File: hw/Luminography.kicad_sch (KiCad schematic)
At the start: 135 parts, among them J1 USB_C_Receptacle_PowerOnly_6P, J2 Conn_01x04, Q1 2N7002, SW1 SW_Push, SW2 SW_Push, U1 LTC4054ES5-4.2, U10 MAX98357AETE+, U100 BH1750FVI-TR, U101 BH1750FVI-TR, U102 BH1750FVI-TR, U103 BH1750FVI-TR, U104 BH1750FVI-TR, U105 BH1750FVI-TR, U106 BH1750FVI-TR, U107 BH1750FVI-TR, U108 BH1750FVI-TR, U109 BH1750FVI-TR, U110 BH1750FVI-TR, U111 BH1750FVI-TR, U112 BH1750FVI-TR, U113 BH1750FVI-TR, U114 BH1750FVI-TR, U115 BH1750FVI-TR, U116 BH1750FVI-TR, U117 BH1750FVI-TR, U118 BH1750FVI-TR, U119 BH1750FVI-TR, U120 BH1750FVI-TR, U121 BH1750FVI-TR, U122 BH1750FVI-TR, U123 BH1750FVI-TR, U2 XS3A1T3157GMX, U200 HD107S, U201 HD107S, U202 HD107S, U203 HD107S, U204 HD107S, U205 HD107S, U206 HD107S, U207 HD107S, U208 HD107S, U209 HD107S, U210 HD107S, U211 HD107S, U212 HD107S, U213 HD107S, U214 HD107S, U215 HD107S, U216 HD107S, U217 HD107S, U218 HD107S, U219 HD107S, U220 HD107S, U221 HD107S, U222 HD107S, U223 HD107S, U3 SPX3819M5-L-3-3, U4 MAX17048G+T10, U5 STM32G030K6Tx, U51 STM32G030C8Tx, U6 ZJY128R-IG01, U7 W25Q16JVUXIQ, U8 BMI270, U9 MMC5603NJ, X1 12.288MHz

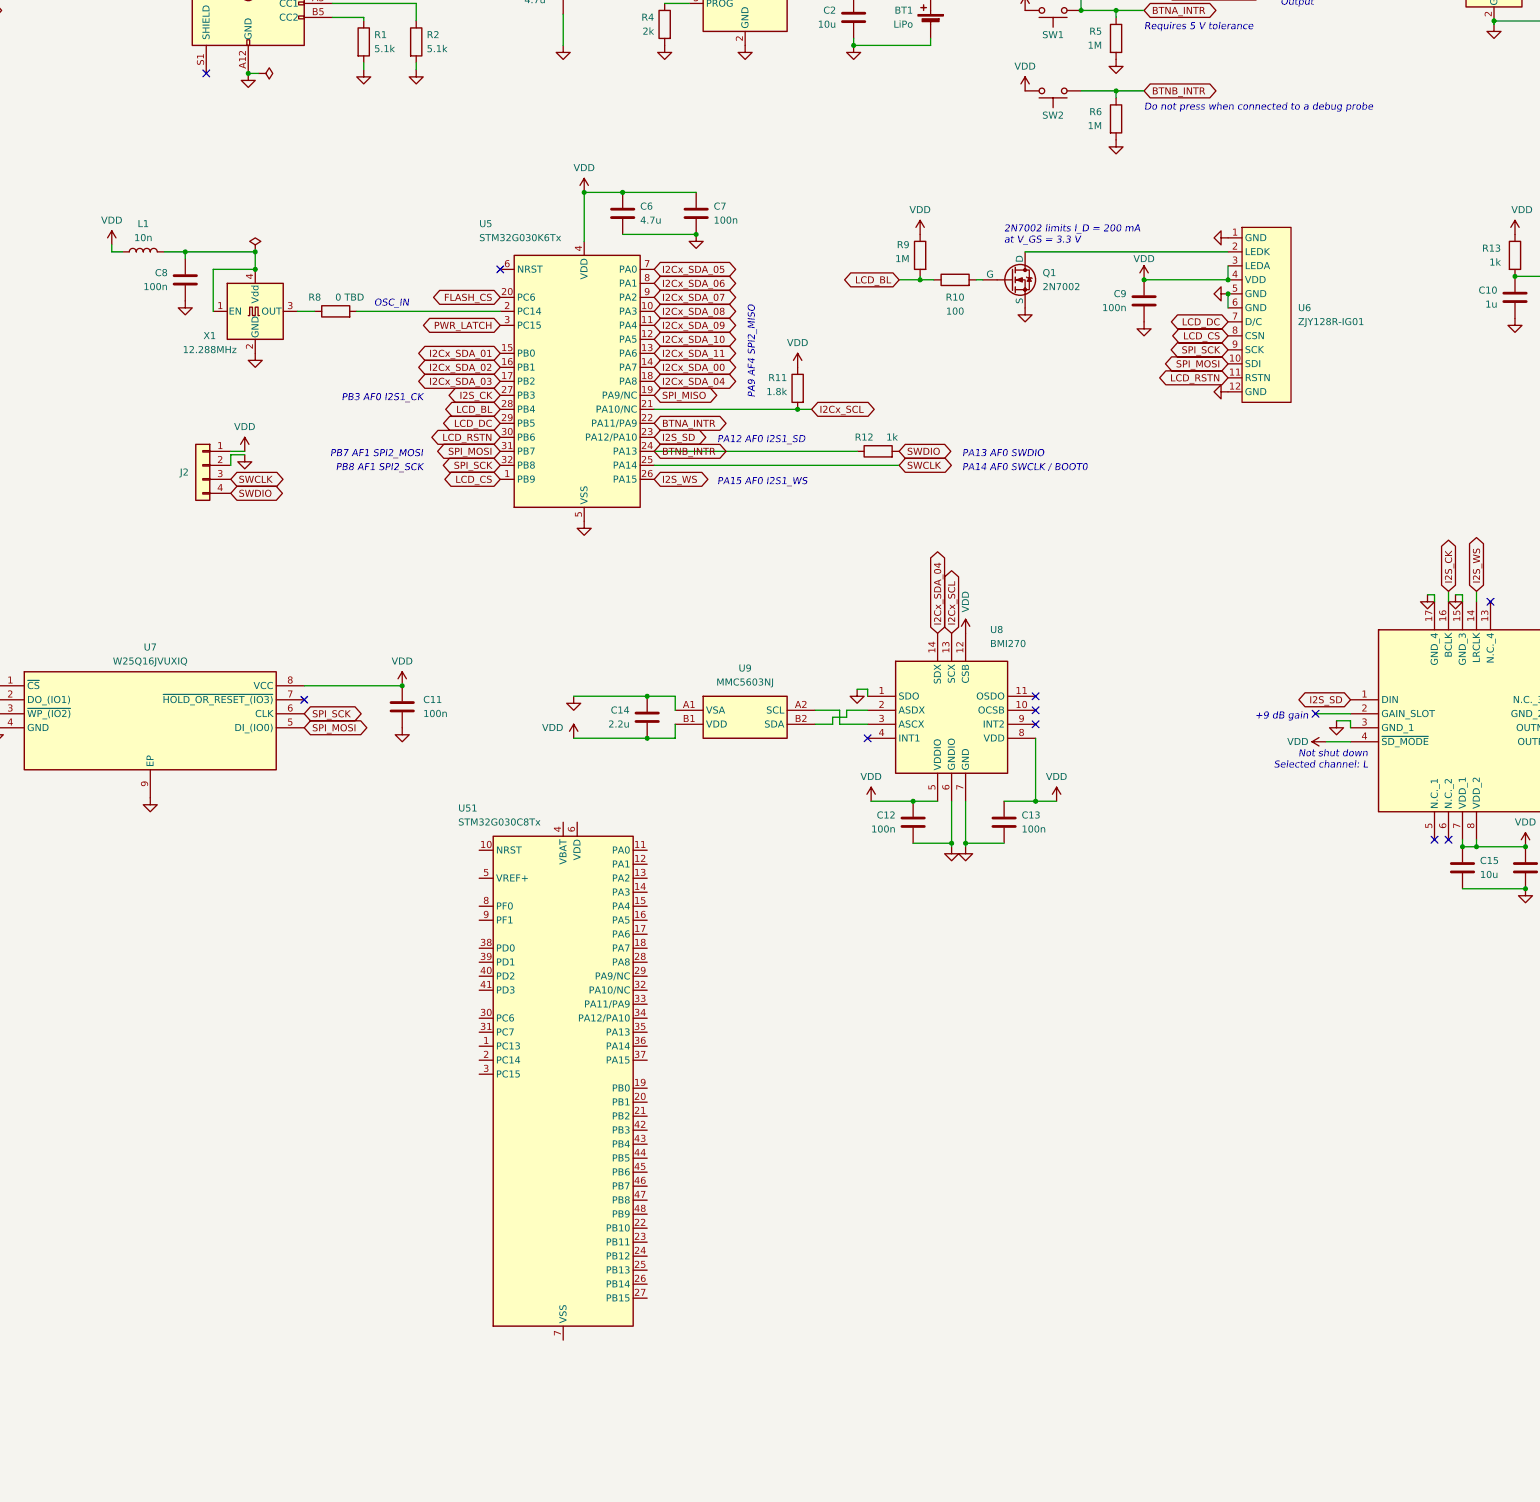
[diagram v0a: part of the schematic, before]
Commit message: Sleep
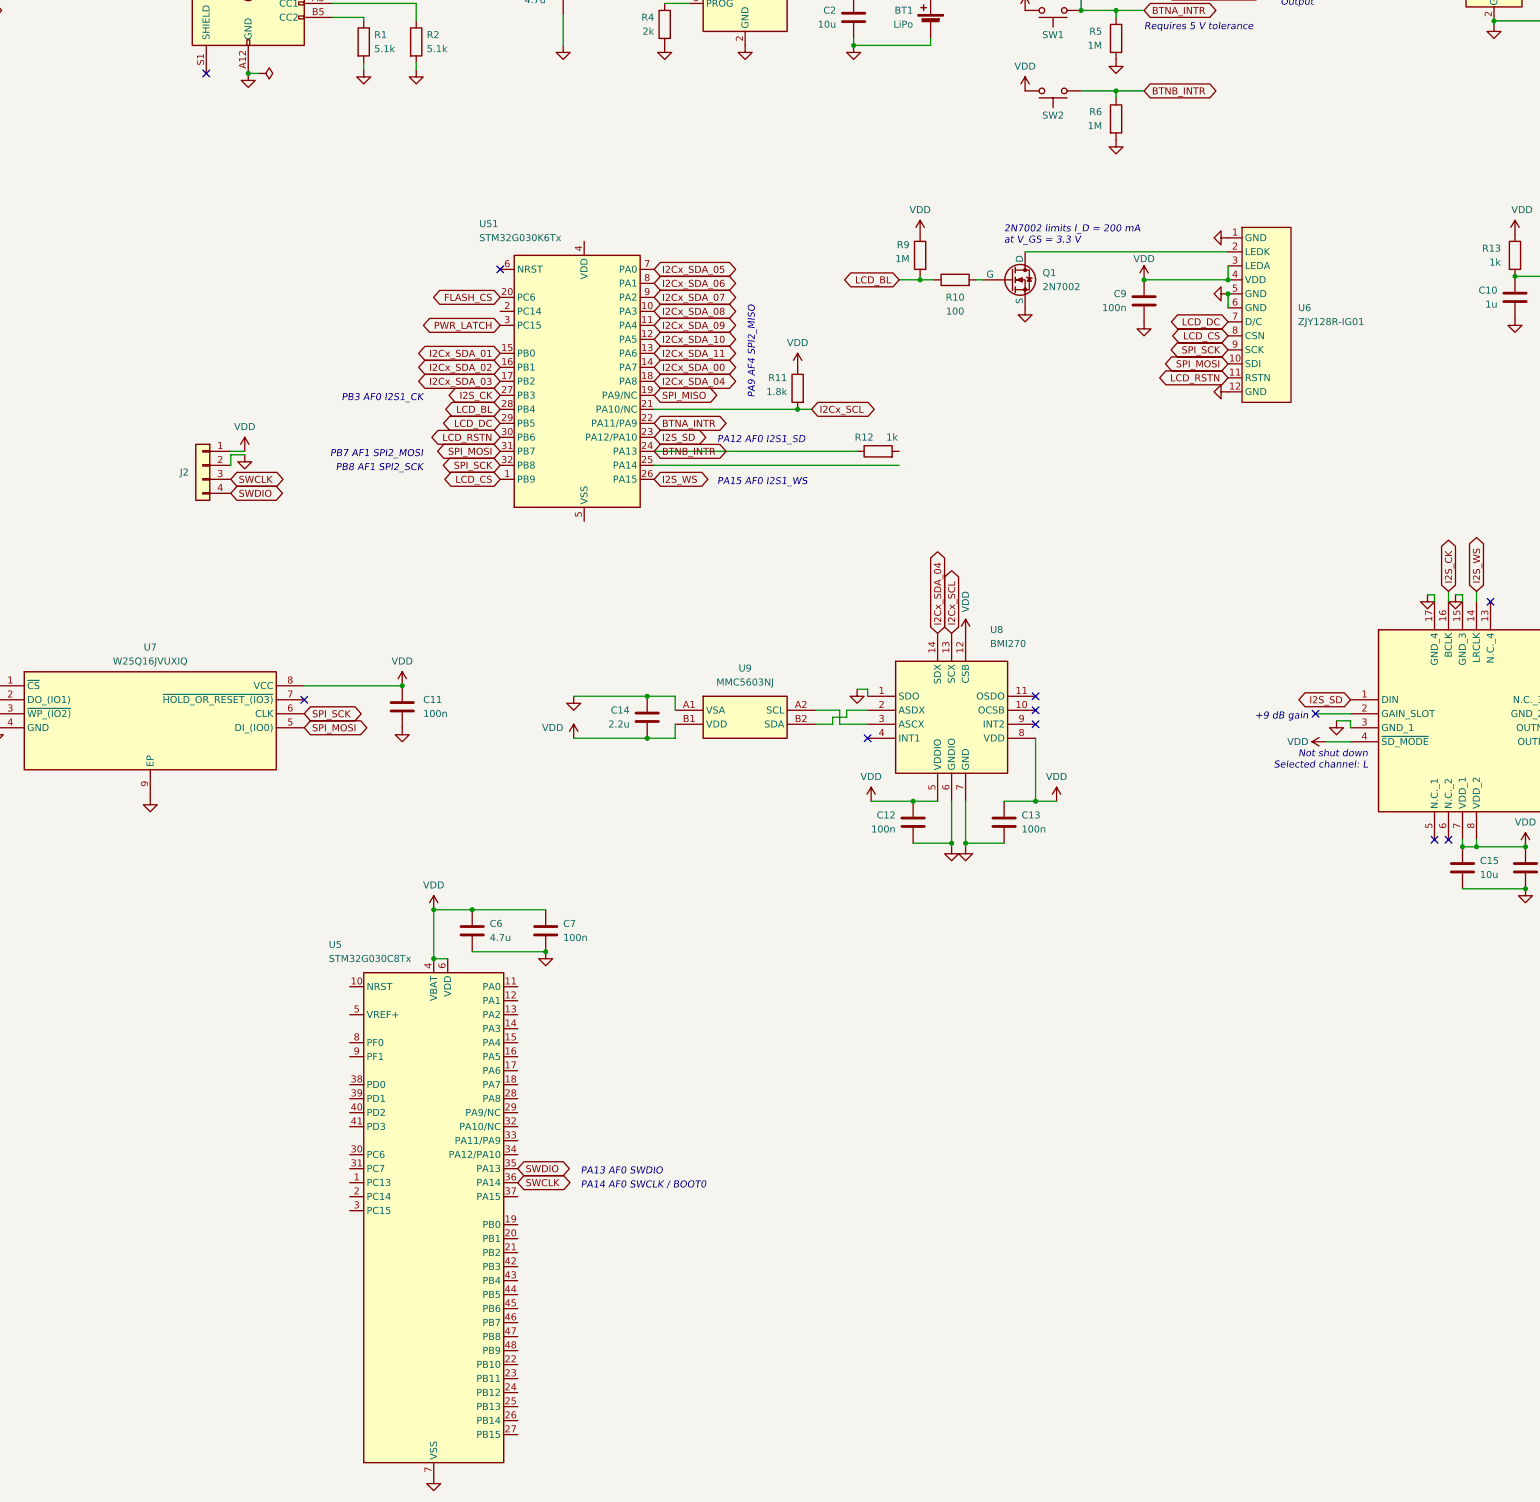
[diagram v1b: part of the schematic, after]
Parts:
- removed C8: 100n, Capacitor_SMD:C_0402_1005Metric, symbol Device:C
- removed L1: 10n, Inductor_SMD:L_0402_1005Metric, symbol Device:L
- removed R8: 0 TBD, Resistor_SMD:R_0402_1005Metric, symbol Device:R
- removed X1: 12.288MHz, Oscillator:Oscillator_SMD_Abracon_ASE-4Pin_3.2x2.5mm, symbol Oscillator:ASE-xxxMHz
- renumbered U51 to U5, U5 to U51
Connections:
- net GND: now also U5.7 (VSS); no longer U51.5 (VSS)
- net SWCLK: now also U5.36 (PA14); no longer U51.25 (PA14)
- net SWDIO: now also U5.35 (PA13); no longer R12.2
- net VDD: now also U5.4 (VBAT), U5.6 (VDD); no longer U51.4 (VDD)
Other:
- note removed: "Do not press when connected to a debug probe"
- note removed: "OSC_IN"
- moved on the sheet: C6, C7, U5

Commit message: 🚧 Finally, add LEDS (board revision WIP)
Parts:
- removed R12: 1k, Resistor_SMD:R_0402_1005Metric, symbol Device:R
- removed U51: STM32G030K6Tx, Package_QFP:LQFP-32_7x7mm_P0.8mm, symbol MCU_ST_STM32G0:STM32G030K6Tx
- added C10, C14, C15: 100n, Capacitor_SMD:C_0402_1005Metric, symbol Device:C
- added C11, C12: 6.8p, Capacitor_SMD:C_0402_1005Metric, symbol Device:C
- added C5, C6: 10u, Capacitor_SMD:C_0402_1005Metric, symbol Device:C
- added L1: 10u, Inductor_SMD:L_Sunlord_SWPA252012S, symbol Device:L
- added R14: 1M, Resistor_SMD:R_0402_1005Metric, symbol Device:R
- added R8: 1.8M, Resistor_SMD:R_0402_1005Metric, symbol Device:R
- added R9: 2.2k, Resistor_SMD:R_0402_1005Metric, symbol Device:R
- added U4: TPS61220DCK, Package_TO_SOT_SMD:Texas_R-PDSO-G6, symbol Regulator_Switching:TPS61220DCK
- added U8: TXS0102DCT, Package_SO:SSOP-8_2.95x2.8mm_P0.65mm, symbol Logic_LevelTranslator:TXS0102DCT
- added Y1: 32MHz 12pF, Crystal:Crystal_SMD_3225-4Pin_3.2x2.5mm, symbol Device:Crystal_GND24
- renumbered C9 to C13, C10 to C16, C11 to C17, C12 to C18, C13 to C19, C14 to C20, C15 to C21, C16 to C22, C5 to C7, C6 to C8, C7 to C9, R9 to R10, R10 to R11, R11 to R12, U9 to U10, U8 to U11, U10 to U12, U4 to U5, U5 to U6, U6 to U7, U7 to U9
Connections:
- net +5V: now also C15.1, C6.1, R8.1, U4.4 (VOUT), U8.7 (VCCB)
- net BTNA_INTR: now also U6.1 (PC13)
- net BTNB_INTR: now also U6.17 (PA6)
- net FLASH_CS: now also U6.30 (PC6)
- net GND: now also C10.2, C11.1, C12.1, C14.2, C15.2, C5.2, C6.2, R14.2, R9.2, U4.3 (GND), U8.2 (GND), Y1.2, Y1.4
- net I2Cx_SCL: now also U6.32 (PA10/NC)
- net I2Cx_SDA_00: now also U6.22 (PB10)
- net I2Cx_SDA_01: now also U6.23 (PB11)
- net I2Cx_SDA_02: now also U6.24 (PB12)
- net I2Cx_SDA_03: now also U6.25 (PB13)
- net I2Cx_SDA_04: now also U6.26 (PB14)
- net I2Cx_SDA_05: now also U6.11 (PA0)
- net I2Cx_SDA_06: now also U6.12 (PA1)
- net I2Cx_SDA_07: now also U6.13 (PA2)
- net I2Cx_SDA_08: now also U6.14 (PA3)
- net I2Cx_SDA_09: now also U6.19 (PB0)
- net I2Cx_SDA_10: now also U6.20 (PB1)
- net I2Cx_SDA_11: now also U6.21 (PB2)
- net I2S_CK: now also U6.42 (PB3)
- net I2S_SD: now also U6.34 (PA12/PA10)
- net I2S_WS: now also U6.37 (PA15)
- net LCD_BL: now also U6.43 (PB4)
- net LCD_CS: now also U6.48 (PB9)
- net LCD_DC: now also U6.44 (PB5)
- net LCD_RSTN: now also U6.45 (PB6)
- net LED_CLK: now also U6.16 (PA5), U8.5 (A1); no longer U217.5 (CI)
- net LED_DATA: now also U6.18 (PA7), U8.4 (A2); no longer U217.6 (DI)
- net PWR_LATCH: now also U6.2 (PC14)
- net SPI_MISO: now also U6.29 (PA9/NC)
- net SPI_MOSI: now also U6.46 (PB7)
- net SPI_SCK: now also U6.47 (PB8)
- net VDD: now also U6.5 (VREF+), C14.1, U8.3 (VCCA)
- net VRI: now also C5.1, L1.1, U4.1 (VIN), U4.6 (EN)
- net at U6.10 (NRST): now also C10.1
- net LSH_OE: now reaches U6.15 (PA4)
- net LSH_OE: now also R14.1, U8.6 (OE)
- net at U6.8 (PF0): now also C11.2, Y1.3
- net at U6.9 (PF1): now also C12.2, Y1.1
- new net: R8.2, R9.1, U4.2 (FB)
- new net: L1.2, U4.5 (L)
- new net LED_CLK_5V: U217.5 (CI), U8.8 (B1)
- new net LED_DATA_5V: U217.6 (DI), U8.1 (B2)
- no-connect marks 17 -> 25
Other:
- note added: "Programmed V_OUT = 4.6 V"
- note added: "V_FB = 500 mV typ."
- moved on the sheet: C17, C18, C19, C20, C7, C8, C9, R12, U10, U11, U5, U6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
